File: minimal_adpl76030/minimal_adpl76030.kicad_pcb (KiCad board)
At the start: 4 copper layers, 15.2 x 15.2 mm, 1 part, among them U1 ADPL76030EUFD-PBF

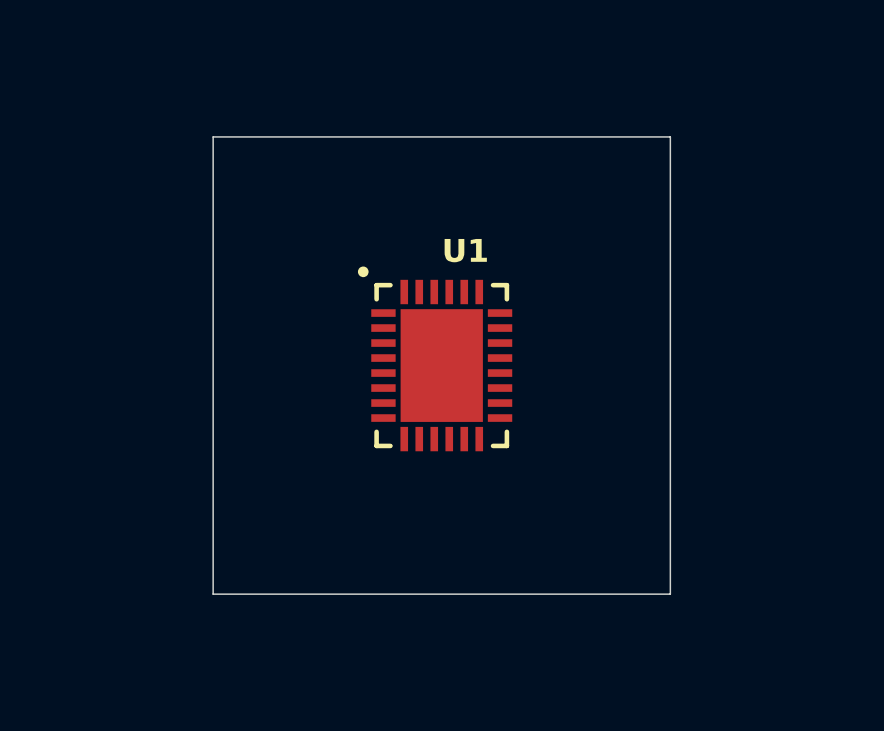
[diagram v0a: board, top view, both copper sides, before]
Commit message: backup
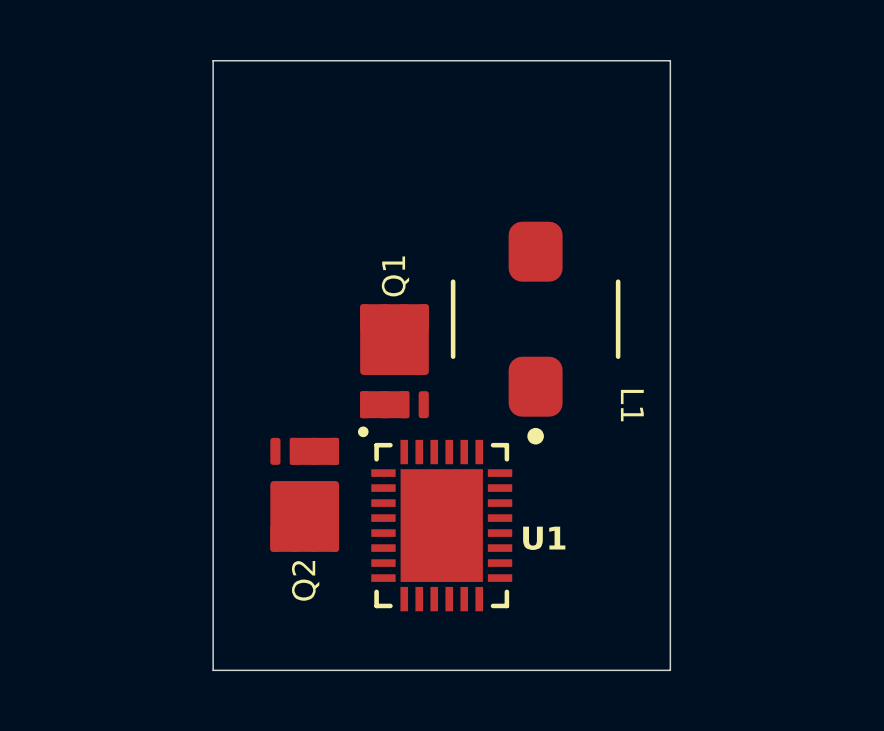
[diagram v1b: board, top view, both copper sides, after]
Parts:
- added L1: 1.0 µH, inductor_footprints:74437336, F.Cu at (143.1, 86.4)
- added Q1: 60 V, transistor_footprints:TSDSON-8FL, F.Cu at (138.4, 87.8)
- added Q2: 60 V, transistor_footprints:TSDSON-8FL, F.Cu at (135.4, 92.2)
- moved U1 5.33 mm to (140.0, 93.3)
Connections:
- U1 pad 1: unconnected-(U1-TG1-Pad1) -> Net-(Q1-G)
- U1 pad 23: unconnected-(U1-SW2-Pad23) -> /SW2
- U1 pad 26: unconnected-(U1-BG1-Pad26) -> /BG1
- U1 pad 28: unconnected-(U1-SW1-Pad28) -> /SW1
- U1 pad 29: unconnected-(U1-GND-Pad29) -> GND
- U1 pad 3: unconnected-(U1-LSN-Pad3) -> Net-(U1-LSN)
- U1 pad 7: unconnected-(U1-TEST1-Pad7) -> GND
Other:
- board size 15.2 x 15.2 mm -> 15.2 x 20.3 mm

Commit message: backup
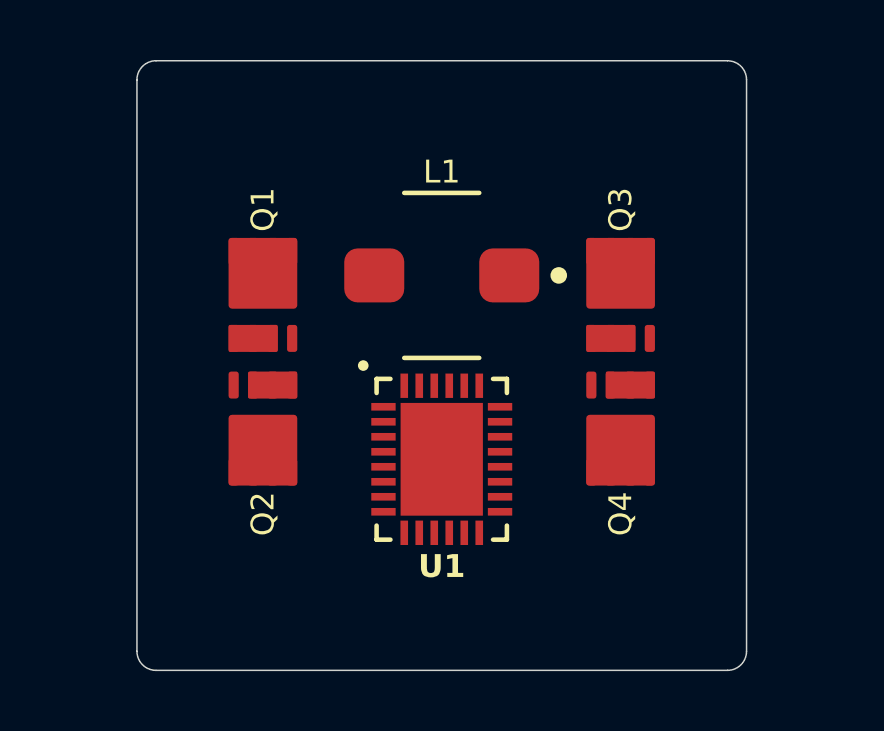
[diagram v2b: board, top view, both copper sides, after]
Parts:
- added Q3: 25 V, transistor_footprints:TSDSON-8FL, F.Cu at (145.9, 85.6)
- added Q4: 25 V, transistor_footprints:TSDSON-8FL, F.Cu at (145.9, 90.0)
- moved Q1 4.91 mm to (134.0, 85.6)
- moved L1 3.45 mm to (140.0, 84.9), turned to 180 degrees
- moved Q2 2.61 mm to (134.0, 90.0)
- moved U1 2.21 mm to (140.0, 91.1)
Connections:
- net Net-(Q1-G) renamed /TG1
- net Net-(U1-LSN) renamed /LSN
- Q1 pad 5: unconnected-(Q1-D-Pad5) -> /VIN
- U1 pad 2: unconnected-(U1-LSP-Pad2) -> /SW1
- U1 pad 21: unconnected-(U1-VOUT-Pad21) -> /VOUT
- U1 pad 22: unconnected-(U1-TG2-Pad22) -> /TG2
- U1 pad 25: unconnected-(U1-BG2-Pad25) -> /BG2
- U1 pad 4: unconnected-(U1-VIN-Pad4) -> /VIN
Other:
- board size 15.2 x 20.3 mm -> 20.3 x 20.3 mm

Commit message: backup
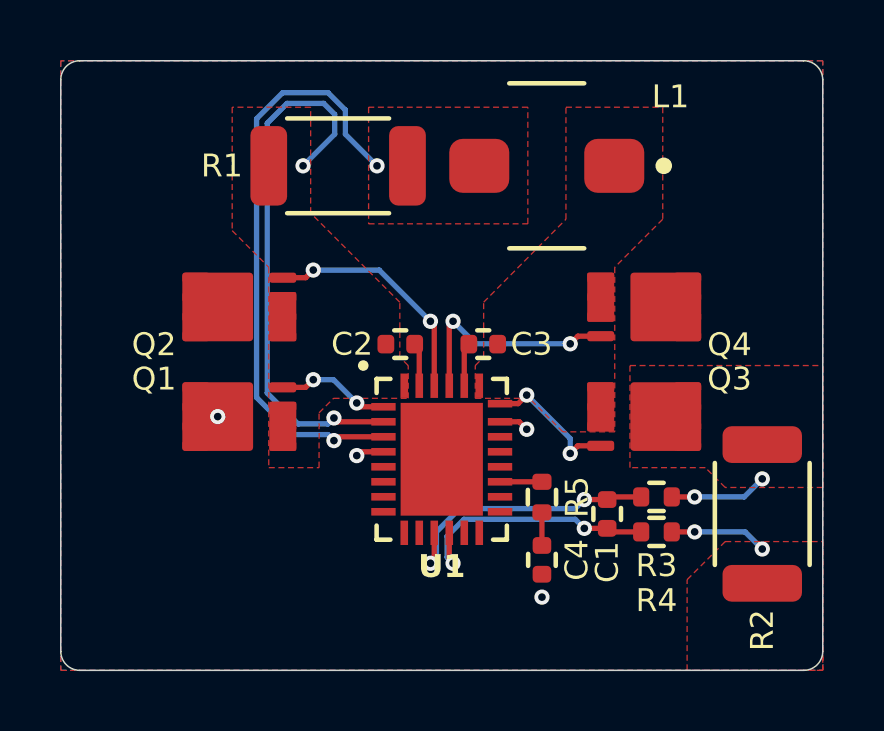
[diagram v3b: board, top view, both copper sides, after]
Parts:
- added C1: 1 µF, capacitor_footprints:C_0402_1005Metric, F.Cu at (145.5, 92.9)
- added C2: 100 nF, capacitor_footprints:C_0402_1005Metric, F.Cu at (138.6, 87.2)
- added C3: 100 nF, capacitor_footprints:C_0402_1005Metric, F.Cu at (141.3, 87.2)
- added C4: 2.2 nF, capacitor_footprints:C_0402_1005Metric, F.Cu at (143.3, 94.4)
- added R1: 0.005 Ω, resistor_footprints:R_2010_5025Metric, F.Cu at (136.5, 81.3)
- added R2: 0.01 Ω, resistor_footprints:R_2010_5025Metric, F.Cu at (150.6, 92.9)
- added R3: 10 kΩ, resistor_footprints:R_0402_1005Metric, F.Cu at (147.1, 92.3)
- added R4: 10 kΩ, resistor_footprints:R_0402_1005Metric, F.Cu at (147.1, 93.5)
- added R5: 10 kΩ, resistor_footprints:R_0402_1005Metric, F.Cu at (143.3, 92.3)
- moved L1 5.06 mm to (143.5, 81.3)
- moved Q1 4.13 mm to (133.2, 89.6), turned to 180 degrees
- moved Q3 4.13 mm to (146.7, 89.6), turned to 0 degrees
- moved Q2 4.13 mm to (133.2, 86.0), turned to 180 degrees
- moved Q4 4.13 mm to (146.7, 86.0), turned to 0 degrees
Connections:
- net /SW1 renamed /LSP
- U1 pad 11: unconnected-(U1-ISP-Pad11) -> /ISP
- U1 pad 12: unconnected-(U1-ISN-Pad12) -> /ISN
- U1 pad 17: unconnected-(U1-VC-Pad17) -> Net-(U1-VC)
- U1 pad 24: unconnected-(U1-BST2-Pad24) -> Net-(U1-BST2)
- U1 pad 27: unconnected-(U1-BST1-Pad27) -> Net-(U1-BST1)
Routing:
- net /LSN: track 0.00 -> 20.0 mm, vias 0 -> 2
- net /LSP: track 0.00 -> 18.3 mm, vias 0 -> 2
- net /ISP: track 0.00 -> 9.51 mm, vias 0 -> 2
- net /ISN: track 0.00 -> 8.93 mm, vias 0 -> 2
- net /BG1: track 0.00 -> 7.93 mm, vias 0 -> 2
- net /BG2: track 0.00 -> 7.54 mm, vias 0 -> 2
- net /TG2: track 0.00 -> 4.67 mm, vias 0 -> 2
- net /VOUT: track 0.00 -> 4.26 mm, vias 0 -> 3
- net /TG1: track 0.00 -> 3.83 mm, vias 0 -> 2
- net /V_OUT: track 0.00 -> 3.25 mm, vias 0 -> 2
- net Net-(U1-BST1): track 0.00 -> 1.45 mm
- net Net-(U1-BST2): track 0.00 -> 1.45 mm
- net Net-(U1-VC): track 0.00 -> 1.40 mm
- net Net-(C4-Pad1): track 0.00 -> 1.10 mm
- net /VIN: track 0.00 -> 0.94 mm, vias 0 -> 2
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- added copper zone on F.Cu, net /LSN
- added copper zone on F.Cu, net /LSP
- added copper zone on F.Cu, net /SW2
- added copper zone on In1.Cu, net /VIN
- added copper zone on F.Cu, net /VOUT
- added copper zone on F.Cu, net /V_OUT
- added copper zone on B.Cu, net GND
- added copper zone on F.Cu, net GND
- added copper zone on In2.Cu, net GND
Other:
- board size 20.3 x 20.3 mm -> 25.4 x 20.3 mm
